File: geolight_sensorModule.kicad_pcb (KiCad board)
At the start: 2 copper layers, 33 x 24.9 mm, 17 parts, among them IC1 ATTINY841-SSU, P1 5V inject, P2 OPEN, P3 IN, P4 OUT, P6 DEBUG, U1 TCRT5000/L, Y1 16Mhz

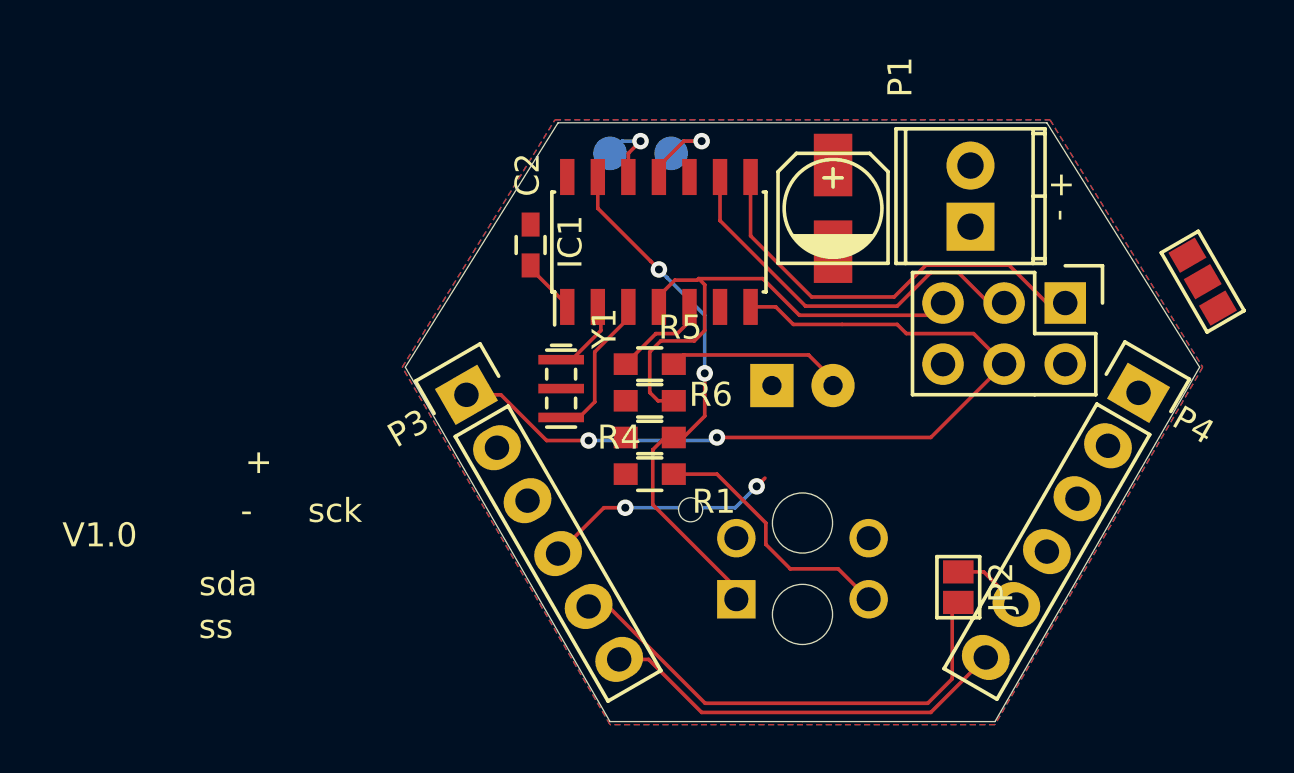
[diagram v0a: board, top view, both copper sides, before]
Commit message: 5mm, rev2 stage (wait a day and finalize)
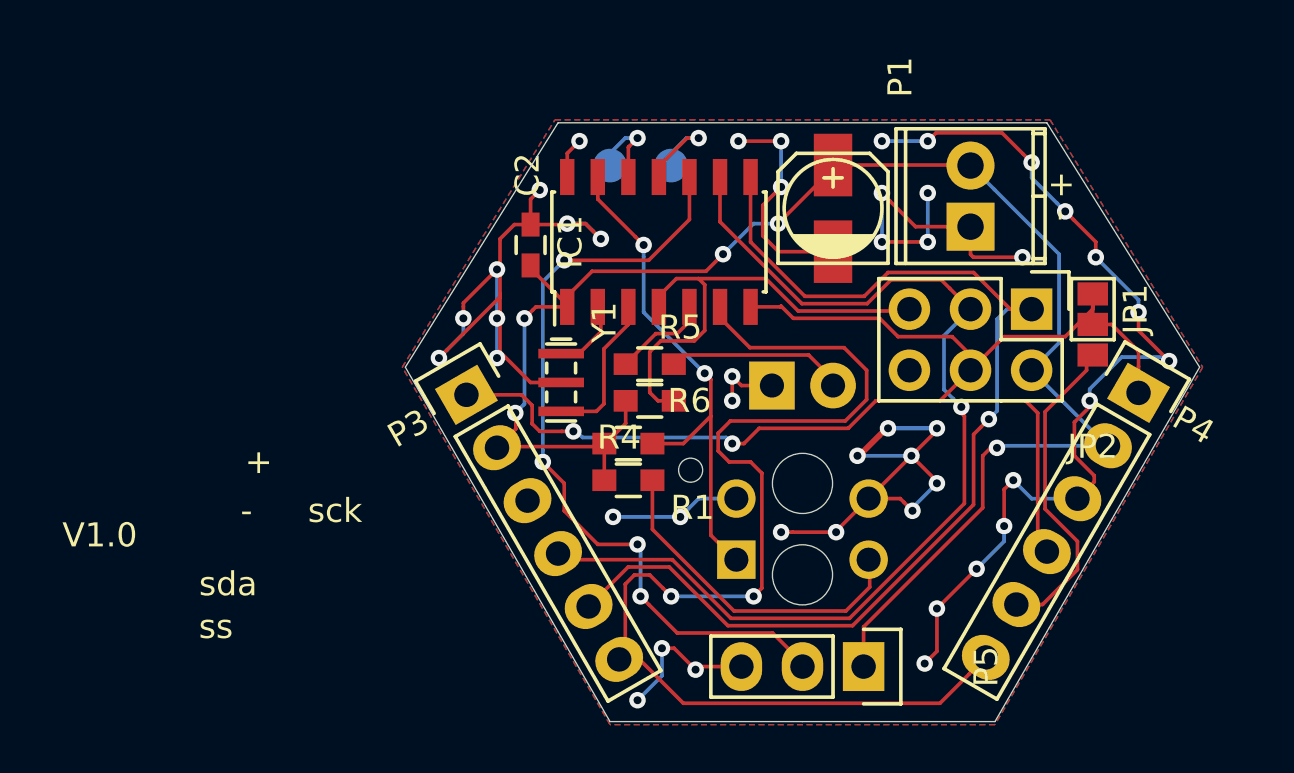
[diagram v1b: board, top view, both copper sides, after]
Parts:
- added P5: AUX Sensor, Pin_Headers:Pin_Header_Straight_1x03, F.Cu at (160.0, 131.1)
- D1: footprint LEDs:LED-8MM -> LEDs:LED-5MM
- JP1: footprint Connect:GS3 -> Connect:GS2
- JP2: footprint Connect:GS2 -> Measurement_Points:Measurement_Point_Square-SMD-Pad_SmallRect
- moved JP2 11.2 mm to (169.5, 118.1), turned to 180 degrees
- moved JP1 4.71 mm to (169.5, 116.2), turned to 0 degrees
- moved U1 1.65 mm to (157.5, 125.3)
- moved P2 1.42 mm to (167.0, 116.2)
- moved R6 0.92 mm to (150.2, 121.8)
- moved R1 0.92 mm to (150.2, 123.3)
- moved P6 0.51 mm to (150.7, 110.2)
- moved Y1 0.25 mm to (147.4, 119.3)
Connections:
- JP1 pad 1: /MISO -> /SDA/MOSI
- JP1 pad 2: Net-(JP1-Pad2) -> /SDA/MOSI
- P4 pad 1: Net-(JP1-Pad2) -> /SDA/MOSI
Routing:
- net GND: track 0.00 -> 129.2 mm, vias 0 -> 45
- net +5V: track 2.35 -> 69.2 mm, vias 0 -> 5
- net /AUX: track 0.00 -> 32.7 mm, vias 0 -> 4
- net /SS: track 17.6 -> 49.5 mm, vias 0 -> 2
- net /SCK/SCL: track 26.1 -> 52.9 mm, vias 2 -> 1
- net Net-(JP2-Pad1): track 2.97 -> 13.4 mm
- net /SDA/MOSI: track 36.0 -> 46.3 mm
- net /MISO: track 38.3 -> 45.9 mm, vias 0 -> 1
- net Net-(R1-Pad2): track 10.8 -> 14.1 mm
- net /RESET: track 21.4 -> 19.5 mm
- net Net-(IC1-Pad13): track 22.2 -> 21.2 mm
